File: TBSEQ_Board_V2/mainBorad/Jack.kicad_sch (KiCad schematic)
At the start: 8 parts

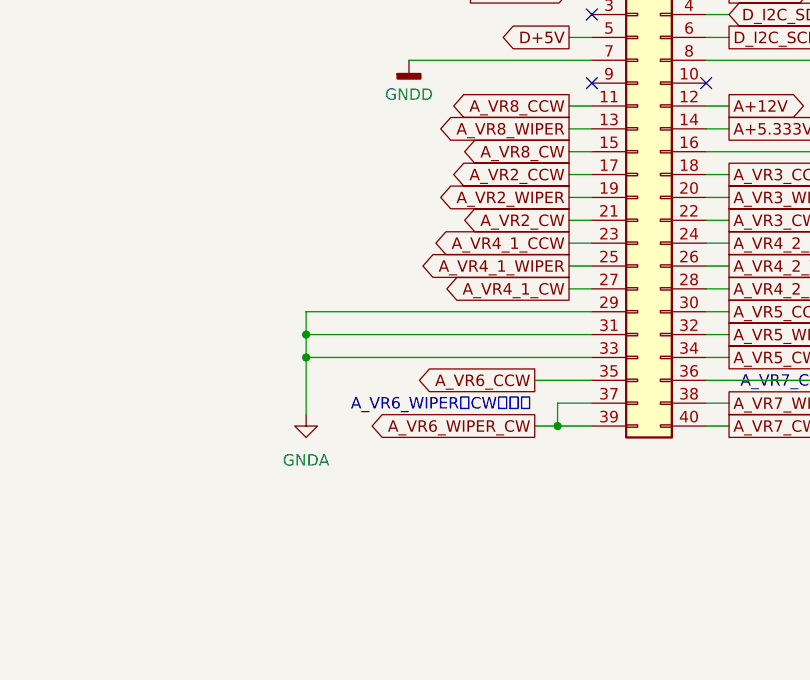
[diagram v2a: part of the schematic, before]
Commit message: mainBoard
VCO
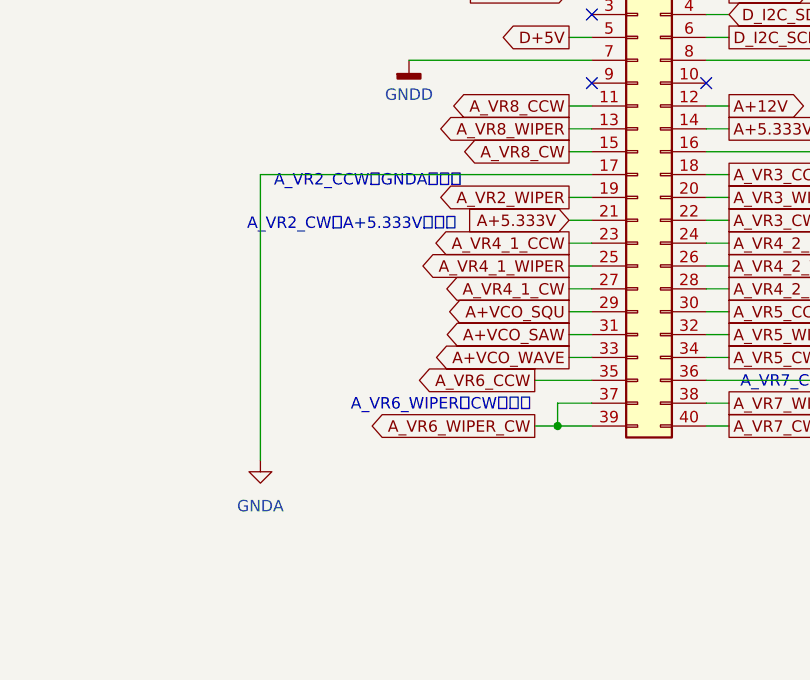
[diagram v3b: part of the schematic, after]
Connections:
- net A_VR2_CCW is gone; now on net GNDA: PanelJ1.17 (Pin_17)
- net A_VR2_CW is gone; now on net A+5.333V: PanelJ1.21 (Pin_21)
- net GNDA: no longer PanelJ1.29 (Pin_29), PanelJ1.31 (Pin_31), PanelJ1.33 (Pin_33)
- new net A+VCO_SAW: PanelJ1.31 (Pin_31)
- new net A+VCO_SQU: PanelJ1.29 (Pin_29)
- new net A+VCO_WAVE: PanelJ1.33 (Pin_33)
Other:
- note added: "A_VR2_CCWはGNDAと接続"
- note added: "A_VR2_CWはA+5.333Vと接続"
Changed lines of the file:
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@@
 	(paper "A4")
-	(junction
-		(at 184.15 80.01)
-		(diameter 0)
-		(color 0 0 0 0)
-	)
 	(junction
 		(at 124.46 91.44)
@@
 	)
 	(junction
-		(at 184.15 77.47)
-		(diameter 0)
-		(color 0 0 0 0)
-	)
-	(junction
 		(at 123.19 31.75)
 		(diameter 0)
@@
 	(wire
 		(pts
+			(xy 213.36 77.47) (xy 215.9 77.47)
+		)
+		(stroke
+			(width 0)
+			(type default)
+		)
+	)
+	(wire
+		(pts
 			(xy 212.09 85.09) (xy 215.9 85.09)
 		)
@@
 	(wire
 		(pts
-			(xy 184.15 80.01) (xy 215.9 80.01)
-		)
-		(stroke
-			(width 0)
-			(type default)
-		)
-	)
-	(wire
-		(pts
-			(xy 215.9 74.93) (xy 184.15 74.93)
-		)
-		(stroke
-			(width 0)
-			(type default)
-		)
-	)
-	(wire
-		(pts
 			(xy 231.14 54.61) (xy 228.6 54.61)
 		)
@@
 	(wire
 		(pts
-			(xy 213.36 59.69) (xy 215.9 59.69)
-		)
-		(stroke
-			(width 0)
-			(type default)
-		)
-	)
-	(wire
-		(pts
 			(xy 135.89 146.05) (xy 129.54 146.05)
 		)
@@
 	(wire
 		(pts
+			(xy 213.36 80.01) (xy 215.9 80.01)
+		)
+		(stroke
+			(width 0)
+			(type default)
+		)
+	)
+	(wire
+		(pts
 			(xy 228.6 69.85) (xy 231.14 69.85)
 		)
@@
 	(wire
 		(pts
-			(xy 184.15 74.93) (xy 184.15 77.47)
-		)
-		(stroke
-			(width 0)
-			(type default)
-		)
-	)
-	(wire
-		(pts
 			(xy 120.65 34.29) (xy 123.19 34.29)
 		)
@@
 	(wire
 		(pts
+			(xy 179.07 59.69) (xy 179.07 91.44)
+		)
+		(stroke
+			(width 0)
+			(type default)
+		)
+	)
+	(wire
+		(pts
 			(xy 120.65 66.04) (xy 124.46 66.04)
 		)
@@
 	(wire
 		(pts
-			(xy 184.15 80.01) (xy 184.15 86.36)
-		)
-		(stroke
-			(width 0)
-			(type default)
-		)
-	)
-	(wire
-		(pts
 			(xy 228.6 74.93) (xy 231.14 74.93)
 		)
@@
 	(wire
 		(pts
-			(xy 184.15 77.47) (xy 215.9 77.47)
-		)
-		(stroke
-			(width 0)
-			(type default)
-		)
-	)
-	(wire
-		(pts
 			(xy 228.6 85.09) (xy 231.14 85.09)
 		)
@@
 	(wire
 		(pts
+			(xy 213.36 74.93) (xy 215.9 74.93)
+		)
+		(stroke
+			(width 0)
+			(type default)
+		)
+	)
+	(wire
+		(pts
 			(xy 228.6 64.77) (xy 231.14 64.77)
 		)
@@
 	(wire
 		(pts
+			(xy 179.07 59.69) (xy 215.9 59.69)
+		)
+		(stroke
+			(width 0)
+			(type default)
+		)
+	)
+	(wire
+		(pts
 			(xy 213.36 57.15) (xy 215.9 57.15)
-		)
-		(stroke
-			(width 0)
-			(type default)
-		)
-	)
-	(wire
-		(pts
-			(xy 184.15 77.47) (xy 184.15 80.01)
 		)
 		(stroke
@@
 		)
 	)
+	(text "A_VR2_CCWはGNDAと接続"
+		(exclude_from_sim no)
+		(at 191.008 60.452 0)
+		(effects
+			(font
+				(size 1.27 1.27)
+			)
+		)
+	)
 	(text "SYNC IN"
 		(exclude_from_sim no)
@@
 		)
 	)
+	(text "A_VR2_CWはA+5.333Vと接続"
+		(exclude_from_sim no)
+		(at 189.23 65.278 0)
+		(effects
+			(font
+				(size 1.27 1.27)
+			)
+		)
+	)
 	(text "A_VR6_WIPERはCWと接続"
 		(exclude_from_sim no)
@@
 		)
 	)
+	(global_label "A+VCO_WAVE"
+		(shape output)
+		(at 213.36 80.01 180)
+		(fields_autoplaced yes)
+		(effects
+			(font
+				(size 1.27 1.27)
+			)
+			(justify right)
+		)
+		(property "Intersheetrefs" "${INTERSHEET_REFS}"
+			(at 198.2795 80.01 0)
+			(effects
+				(font
+					(size 1.27 1.27)
+				)
+				(justify right)
+				(hide yes)
+			)
+		)
+	)
 	(global_label "D_I2C_SCL"
 		(shape output)
@@
 		)
 	)
-	(global_label "A_VR2_CCW"
-		(shape output)
-		(at 213.36 59.69 180)
-		(fields_autoplaced yes)
-		(effects
-			(font
-				(size 1.27 1.27)
-			)
-			(justify right)
-		)
-		(property "Intersheetrefs" "${INTERSHEET_REFS}"
-			(at 199.7915 59.69 0)
+	(global_label "A+VCO_SAW"
+		(shape output)
+		(at 213.36 77.47 180)
+		(fields_autoplaced yes)
+		(effects
+			(font
+				(size 1.27 1.27)
+			)
+			(justify right)
+		)
+		(property "Intersheetrefs" "${INTERSHEET_REFS}"
+			(at 199.3076 77.47 0)
 			(effects
 				(font
@@
 		)
 	)
+	(global_label "A+5.333V"
+		(shape input)
+		(at 213.36 64.77 180)
+		(fields_autoplaced yes)
+		(effects
+			(font
+				(size 1.27 1.27)
+			)
+			(justify right)
+		)
+		(property "Intersheetrefs" "${INTERSHEET_REFS}"
+			(at 201.1824 64.77 0)
+			(effects
+				(font
+					(size 1.27 1.27)
+				)
+				(justify right)
+				(hide yes)
+			)
+		)
+	)
 	(global_label "A+12V"
 		(shape output)
@@
 		(property "Intersheetrefs" "${INTERSHEET_REFS}"
 			(at 205.2343 44.45 0)
-			(effects
-				(font
-					(size 1.27 1.27)
-				)
-				(justify right)
-				(hide yes)
-			)
-		)
-	)
-	(global_label "A_VR2_CW"
-		(shape output)
-		(at 213.36 64.77 180)
-		(fields_autoplaced yes)
-		(effects
-			(font
-				(size 1.27 1.27)
-			)
-			(justify right)
-		)
-		(property "Intersheetrefs" "${INTERSHEET_REFS}"
-			(at 201.0615 64.77 0)
 			(effects
 				(font
@@
 		(property "Intersheetrefs" "${INTERSHEET_REFS}"
 			(at 96.1352 140.97 0)
+			(effects
+				(font
+					(size 1.27 1.27)
+				)
+				(justify right)
+				(hide yes)
+			)
+		)
+	)
+	(global_label "A+VCO_SQU"
+		(shape output)
+		(at 213.36 74.93 180)
+		(fields_autoplaced yes)
+		(effects
+			(font
+				(size 1.27 1.27)
+			)
+			(justify right)
+		)
+		(property "Intersheetrefs" "${INTERSHEET_REFS}"
+			(at 199.1866 74.93 0)
 			(effects
 				(font
@@
 	)
 	(symbol
-		(lib_id "power:GNDA")
-		(at 184.15 86.36 0)
-		(unit 1)
-		(exclude_from_sim no)
-		(in_bom yes)
-		(on_board yes)
-		(dnp no)
-		(fields_autoplaced yes)
-		(property "Reference" "#PWR025"
-			(at 184.15 92.71 0)
-			(effects
-				(font
-					(size 1.27 1.27)
-				)
-				(hide yes)
-			)
-		)
-		(property "Value" "GNDA"
-			(at 184.15 91.44 0)
-			(effects
-				(font
-					(size 1.27 1.27)
-				)
-			)
-		)
-		(property "Footprint" ""
-			(at 184.15 86.36 0)
-			(effects
-				(font
-					(size 1.27 1.27)
-				)
-				(hide yes)
-			)
-		)
-		(property "Datasheet" ""
-			(at 184.15 86.36 0)
-			(effects
-				(font
-					(size 1.27 1.27)
-				)
-				(hide yes)
-			)
-		)
-		(property "Description" "Power symbol creates a global label with name \"GNDA\" , analog ground"
-			(at 184.15 86.36 0)
-			(effects
-				(font
-					(size 1.27 1.27)
-				)
-				(hide yes)
-			)
-		)
-		(pin "1"
-		)
-		(instances
-			(project "mainBorad"
-				(path "/74b57c73-2ea6-4d1a-baa5-ad46186fbb51/0ae150e0-c08a-4733-b66b-e4b7868d24b7"
-					(reference "#PWR025")
-					(unit 1)
-				)
-			)
-		)
-	)
-	(symbol
 		(lib_id "Connector_Generic:Conn_01x03")
 		(at 140.97 143.51 0)
@@
 					(unit 1)
 				)
+			)
+		)
+	)
+	(symbol
+		(lib_id "power:GNDA")
+		(at 179.07 91.44 0)
+		(unit 1)
+		(exclude_from_sim no)
+		(in_bom yes)
+		(on_board yes)
+		(dnp no)
+		(fields_autoplaced yes)
+		(property "Reference" "#PWR025"
+			(at 179.07 97.79 0)
+			(effects
+				(font
+					(size 1.27 1.27)
+				)
+				(hide yes)
+			)
+		)
+		(property "Value" "GNDA"
+			(at 179.07 96.52 0)
+			(effects
+				(font
+					(size 1.27 1.27)
+				)
+			)
+		)
+		(property "Footprint" ""
+			(at 179.07 91.44 0)
+			(effects
+				(font
+					(size 1.27 1.27)
+				)
+				(hide yes)
+			)
+		)
+		(property "Datasheet" ""
+			(at 179.07 91.44 0)
+			(effects
+				(font
+					(size 1.27 1.27)
+				)
+				(hide yes)
+			)
+		)
+		(property "Description" "Power symbol creates a global label with name \"GNDA\" , analog ground"
+			(at 179.07 91.44 0)
+			(effects
+				(font
+					(size 1.27 1.27)
+				)
+				(hide yes)
+			)
+		)
+		(pin "1"
+		)
+		(instances
+			(project "mainBorad"
+				(path "/74b57c73-2ea6-4d1a-baa5-ad46186fbb51/0ae150e0-c08a-4733-b66b-e4b7868d24b7"
+					(reference "#PWR025")
+					(unit 1)
+				)
